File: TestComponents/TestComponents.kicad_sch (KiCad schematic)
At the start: 19 parts, among them J3V1 Conn_01x01_Male, J5 RFShield_OnePiece, J6 RFShield_OnePiece, U1 AD7991, U1 LCC110, U2 ADS1219

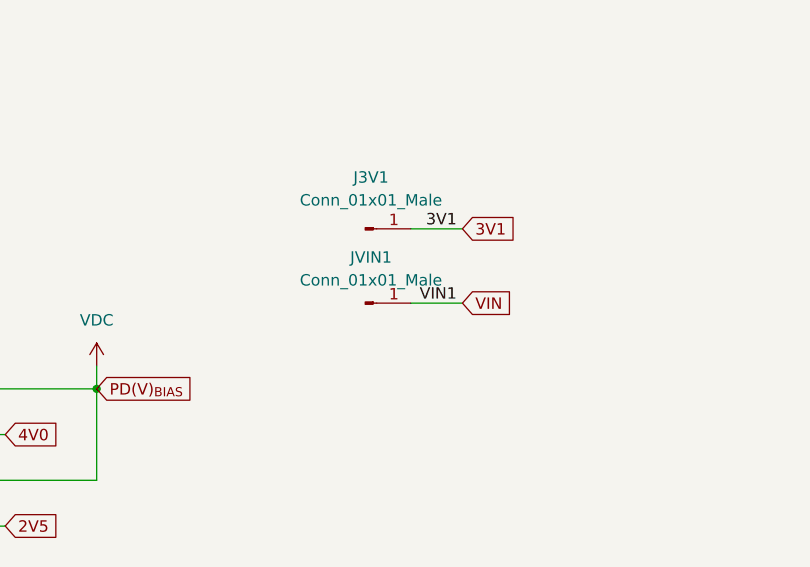
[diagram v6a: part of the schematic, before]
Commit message: SpectDrone Development
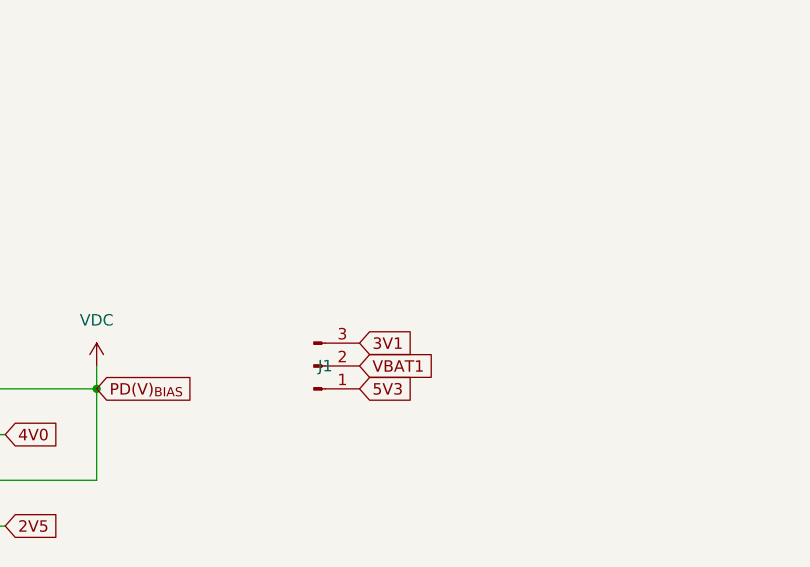
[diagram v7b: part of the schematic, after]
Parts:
- removed J3V1, JVIN1: Conn_01x01_Male, Connector_PinHeader_2.54mm:PinHeader_1x01_P2.54mm_Vertical, symbol Connector:Conn_01x01_Male
- added J1: Conn_01x03_Socket, Connector_PinHeader_2.54mm:PinHeader_1x03_P2.54mm_Vertical, symbol Connector:Conn_01x03_Pin
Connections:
- net 3V1: now also J1.3 (Pin_3)
- net 5V3: now also J1.1 (Pin_1)
- new net VBAT1: J1.2 (Pin_2)
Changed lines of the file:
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@@
-    (stroke (width 0) (type default))
-  )
-  (wire (pts (xy 137.16 106.045) (xy 131.445 106.045))
-    (stroke (width 0) (type default))
-  )
-  (wire (pts (xy 137.16 114.3) (xy 131.445 114.3))
     (stroke (width 0) (type default))
   )
@@
     (effects (font (size 1.27 1.27)) (justify left bottom))
   )
-  (label "3V1" (at 136.525 106.045 180) (fields_autoplaced)
-    (effects (font (size 1.27 1.27)) (justify right bottom))
-  )
   (label "SCL_{RF}" (at 200.66 141.605 0) (fields_autoplaced)
     (effects (font (size 1.27 1.27)) (justify left bottom))
@@
     (effects (font (size 1.27 1.27)) (justify right bottom))
   )
-  (label "VIN1" (at 136.525 114.3 180) (fields_autoplaced)
-    (effects (font (size 1.27 1.27)) (justify right bottom))
-  )
   (label "GND1" (at 104.14 40.64 180) (fields_autoplaced)
     (effects (font (size 1.27 1.27)) (justify right bottom))
@@
     )
   )
+  (global_label "5V3" (shape input) (at 125.73 123.825 0) (fields_autoplaced)
+    (effects (font (size 1.27 1.27)) (justify left))
+    (property "Intersheetrefs" "${INTERSHEET_REFS}" (at 132.2228 123.825 0)
+      (effects (font (size 1.27 1.27)) (justify left) hide)
+    )
+  )
   (global_label "S2_{RF}" (shape input) (at 141.605 38.735 180) (fields_autoplaced)
     (effects (font (size 1.27 1.27)) (justify right))
@@
     )
   )
-  (global_label "3V1" (shape input) (at 137.16 106.045 0) (fields_autoplaced)
-    (effects (font (size 1.27 1.27)) (justify left))
-    (property "Intersheetrefs" "${INTERSHEET_REFS}" (at 143.0807 105.9656 0)
+  (global_label "3V1" (shape input) (at 125.73 118.745 0) (fields_autoplaced)
+    (effects (font (size 1.27 1.27)) (justify left))
+    (property "Intersheetrefs" "${INTERSHEET_REFS}" (at 131.6507 118.6656 0)
       (effects (font (size 1.27 1.27)) (justify left) hide)
     )
@@
     )
   )
-  (global_label "VIN" (shape input) (at 137.16 114.3 0) (fields_autoplaced)
-    (effects (font (size 1.27 1.27)) (justify left))
-    (property "Intersheetrefs" "${INTERSHEET_REFS}" (at 142.5969 114.2206 0)
-      (effects (font (size 1.27 1.27)) (justify left) hide)
-    )
-  )
   (global_label "5V3" (shape input) (at 196.215 87.63 180) (fields_autoplaced)
     (effects (font (size 1.27 1.27)) (justify right))
@@
     (property "Intersheetrefs" "${INTERSHEET_REFS}" (at 191.3224 100.8856 0)
       (effects (font (size 1.27 1.27)) (justify right) hide)
+    )
+  )
+  (global_label "VBAT1" (shape input) (at 125.73 121.285 0) (fields_autoplaced)
+    (effects (font (size 1.27 1.27)) (justify left))
+    (property "Intersheetrefs" "${INTERSHEET_REFS}" (at 134.3395 121.285 0)
+      (effects (font (size 1.27 1.27)) (justify left) hide)
     )
   )
@@
         (path "/e63e39d7-6ac0-4ffd-8aa3-1841a4541b55"
           (reference "C38") (unit 1)
-        )
-      )
-    )
-  )
-  (symbol (lib_id "Connector:Conn_01x01_Male") (at 126.365 106.045 0) (unit 1)
-    (in_bom no) (on_board yes) (dnp no) (fields_autoplaced)
-    (property "Reference" "J3V1" (at 127 100.33 0)
-      (effects (font (size 1.27 1.27)))
-    )
-    (property "Value" "Conn_01x01_Male" (at 127 102.87 0)
-      (effects (font (size 1.27 1.27)))
-    )
-    (property "Footprint" "Connector_PinHeader_2.54mm:PinHeader_1x01_P2.54mm_Vertical" (at 126.365 106.045 0)
-      (effects (font (size 1.27 1.27)) hide)
-    )
-    (property "Datasheet" "~" (at 126.365 106.045 0)
-      (effects (font (size 1.27 1.27)) hide)
-    )
-    (property "Part Number" "PH1-01-UA" (at 126.365 106.045 0)
-      (effects (font (size 1.27 1.27)) hide)
-    )
-    (pin "1")
-    (instances
-      (project "TestComponents"
-        (path "/e63e39d7-6ac0-4ffd-8aa3-1841a4541b55"
-          (reference "J3V1") (unit 1)
         )
       )
@@
         (path "/e63e39d7-6ac0-4ffd-8aa3-1841a4541b55"
           (reference "C1") (unit 1)
+        )
+      )
+    )
+  )
+  (symbol (lib_id "Connector:Conn_01x03_Pin") (at 120.65 121.285 0) (mirror x) (unit 1)
+    (in_bom no) (on_board yes) (dnp no)
+    (property "Reference" "J1" (at 121.92 121.285 0)
+      (effects (font (size 1.27 1.27)))
+    )
+    (property "Value" "Conn_01x03_Socket" (at 120.015 115.57 0)
+      (effects (font (size 1.27 1.27)) hide)
+    )
+    (property "Footprint" "Connector_PinHeader_2.54mm:PinHeader_1x03_P2.54mm_Vertical" (at 120.65 121.285 0)
+      (effects (font (size 1.27 1.27)) hide)
+    )
+    (property "Datasheet" "~" (at 120.65 121.285 0)
+      (effects (font (size 1.27 1.27)) hide)
+    )
+    (pin "1")
+    (pin "2")
+    (pin "3")
+    (instances
+      (project "TestComponents"
+        (path "/e63e39d7-6ac0-4ffd-8aa3-1841a4541b55"
+          (reference "J1") (unit 1)
         )
       )
@@
         )
       )
-    )
-  )
-  (symbol (lib_id "Connector:Conn_01x01_Male") (at 126.365 114.3 0) (unit 1)
-    (in_bom no) (on_board yes) (dnp no) (fields_autoplaced)
-    (property "Reference" "JVIN1" (at 127 109.22 0)
-      (effects (font (size 1.27 1.27)))
-    )
-    (property "Value" "Conn_01x01_Male" (at 127 111.76 0)
-      (effects (font (size 1.27 1.27)))
-    )
-    (property "Footprint" "Connector_PinHeader_2.54mm:PinHeader_1x01_P2.54mm_Vertical" (at 126.365 114.3 0)
-      (effects (font (size 1.27 1.27)) hide)
-    )
-    (property "Datasheet" "~" (at 126.365 114.3 0)
-      (effects (font (size 1.27 1.27)) hide)
-    )
-    (property "Part Number" "PH1-01-UA" (at 126.365 114.3 0)
-      (effects (font (size 1.27 1.27)) hide)
-    )
-    (pin "1")
-    (instances
-      (project "TestComponents"
-        (path "/e63e39d7-6ac0-4ffd-8aa3-1841a4541b55"
-          (reference "JVIN1") (unit 1)
-        )
-      )
